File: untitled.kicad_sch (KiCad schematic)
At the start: 11 parts, among them J4 691313510002, U5 TLV1117LV33DCYT

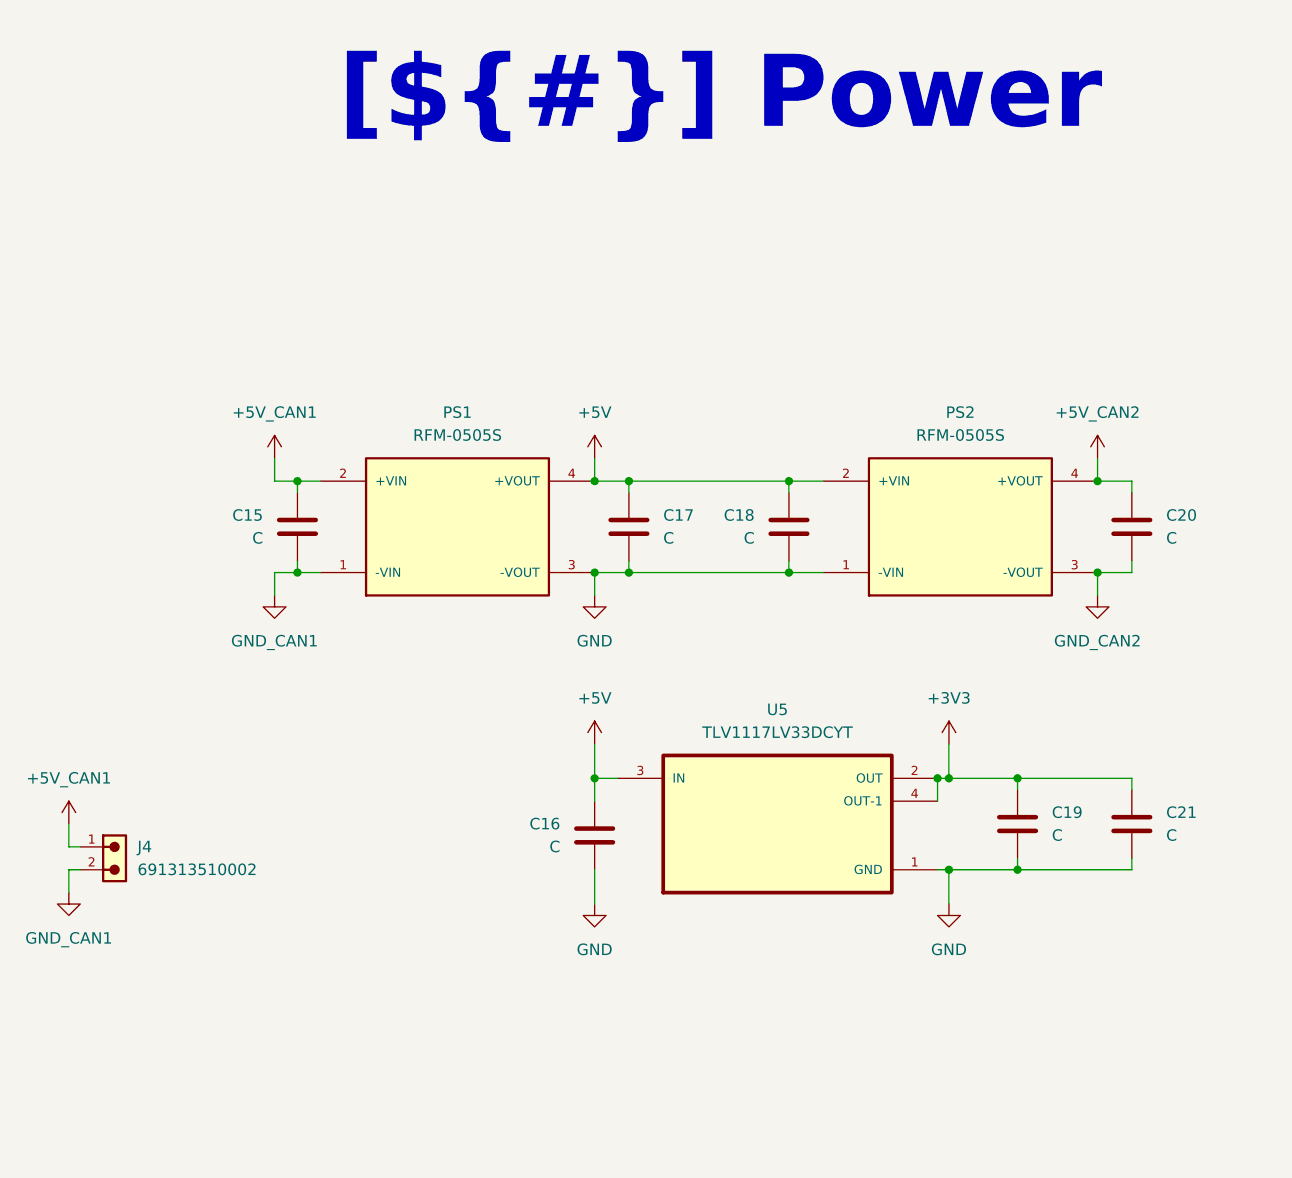
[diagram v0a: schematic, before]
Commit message: Final Changes, Updated to Checked
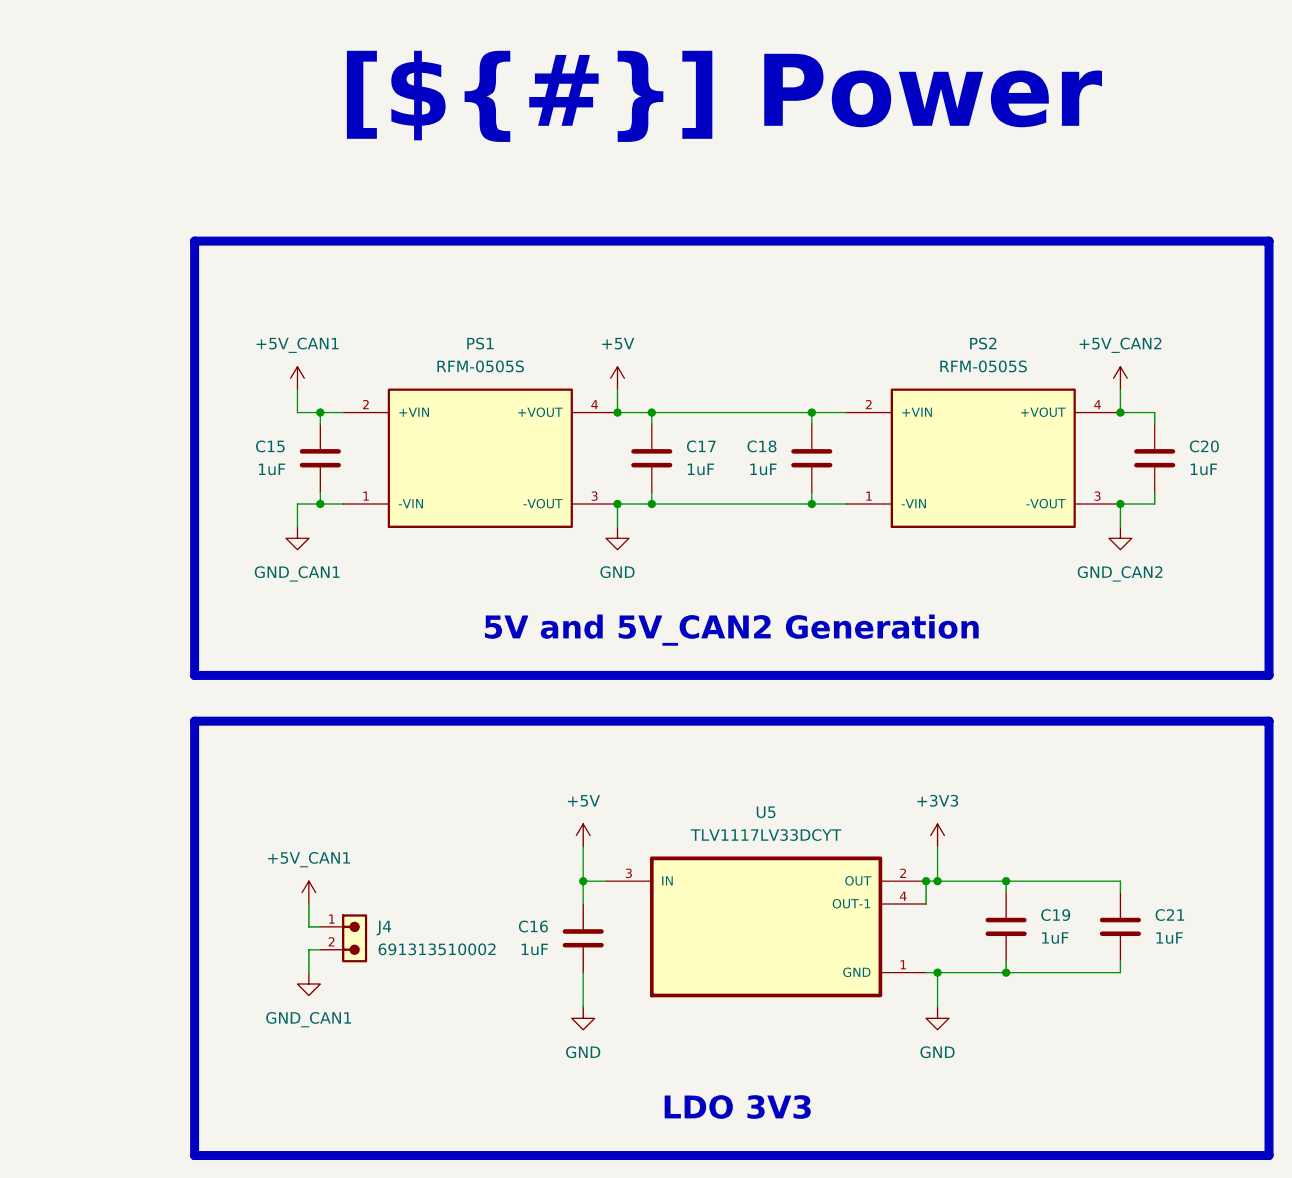
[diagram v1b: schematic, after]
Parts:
- C15, C16, C17, C18, C19, C20, C21: value C -> 1uF
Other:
- moved on the sheet: C15, C16, C17, C18, C19, C20, C21, J4, PS1, PS2, U5
